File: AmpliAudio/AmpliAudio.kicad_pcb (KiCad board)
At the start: 2 copper layers, 110 x 100 mm, 52 parts, among them J2 Conn_01x02, J3 Conn_01x03, Q1 2N2907, Q10 TIP32, Q11 BD138, Q12 TIP31, Q13 2N2222, Q2 2N2907, Q3 2N2907, Q4 2N2222, Q5 2N2222, Q6 2N2907, Q7 2N2907, Q8 BD139, Q9 BD139, U1 Relay_1CT, U2 Jack_Mono

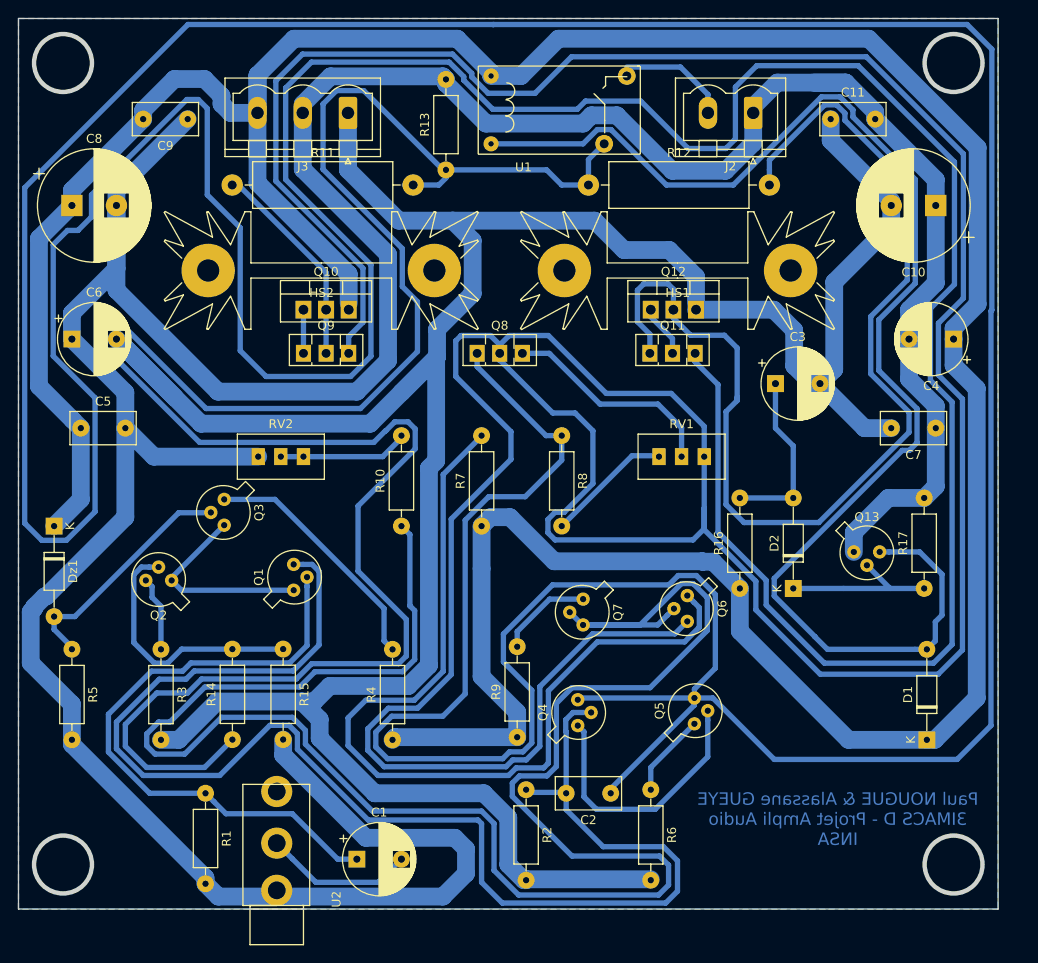
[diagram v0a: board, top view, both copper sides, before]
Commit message: Version Finale
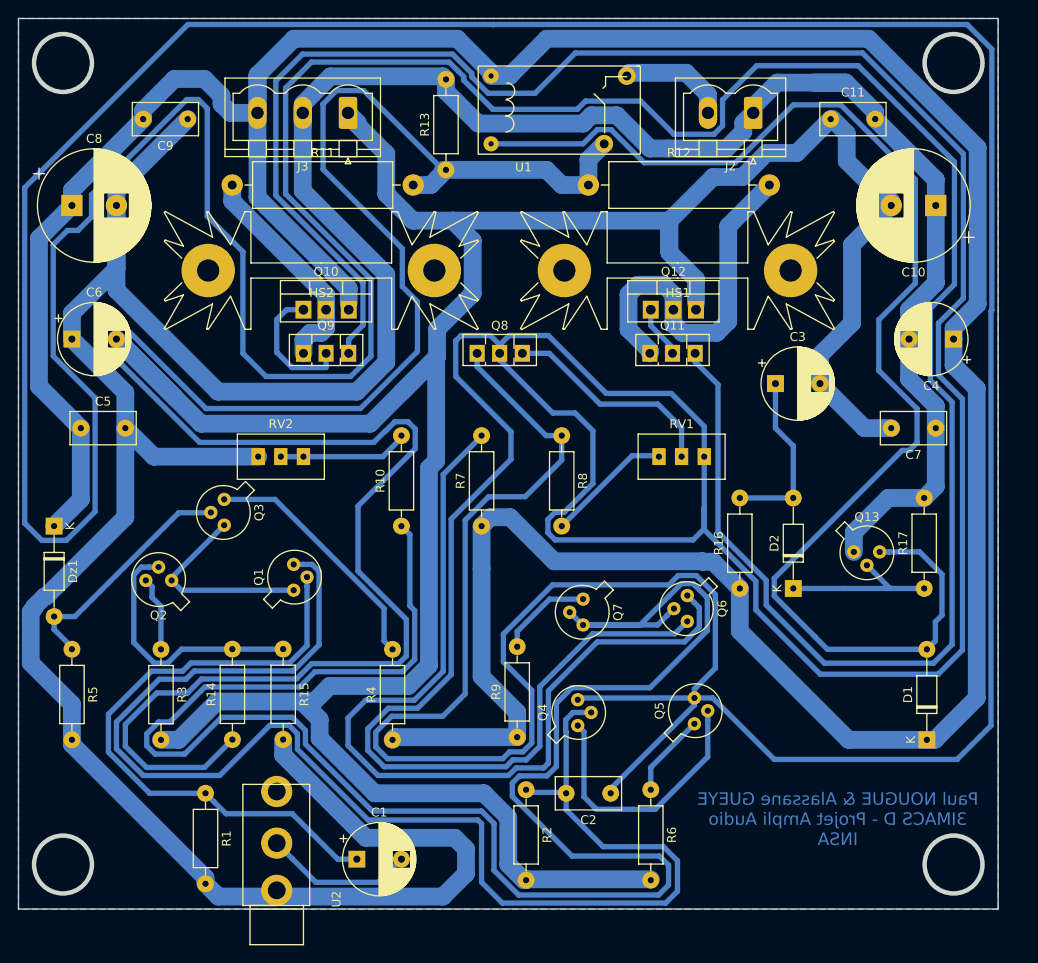
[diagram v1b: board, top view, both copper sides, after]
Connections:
- Q9 pad 1: Net-(Q10-Pad1) -> Net-(Q10-Pad2)
- Q9 pad 2: Net-(Q10-Pad2) -> Net-(Q10-Pad1)
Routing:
- net Net-(Q11-Pad1): track 124.2 -> 40.7 mm
- net Net-(Q10-Pad1): track 5.00 -> 15.0 mm
- net -12V: track 313.9 -> 323.0 mm
- net Net-(D1-Pad2): track 153.5 -> 150.2 mm
- net Net-(C2-Pad1): track 787.6 -> 784.5 mm
- net Net-(Q10-Pad2): track 23.1 -> 25.1 mm
- net GND: track 405.2 -> 403.5 mm
- net Net-(R11-Pad2): track 244.8 -> 243.3 mm
- net Net-(Q6-Pad3): track 417.9 -> 418.9 mm
